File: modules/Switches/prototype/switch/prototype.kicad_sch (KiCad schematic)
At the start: 22 parts, among them J1 Conn_01x09, Q1 J109/J112, Q2 J109/J112, Q3 2N3906, SW2 SW_Push_LED, U1 TL072, U2 SN74HCS74

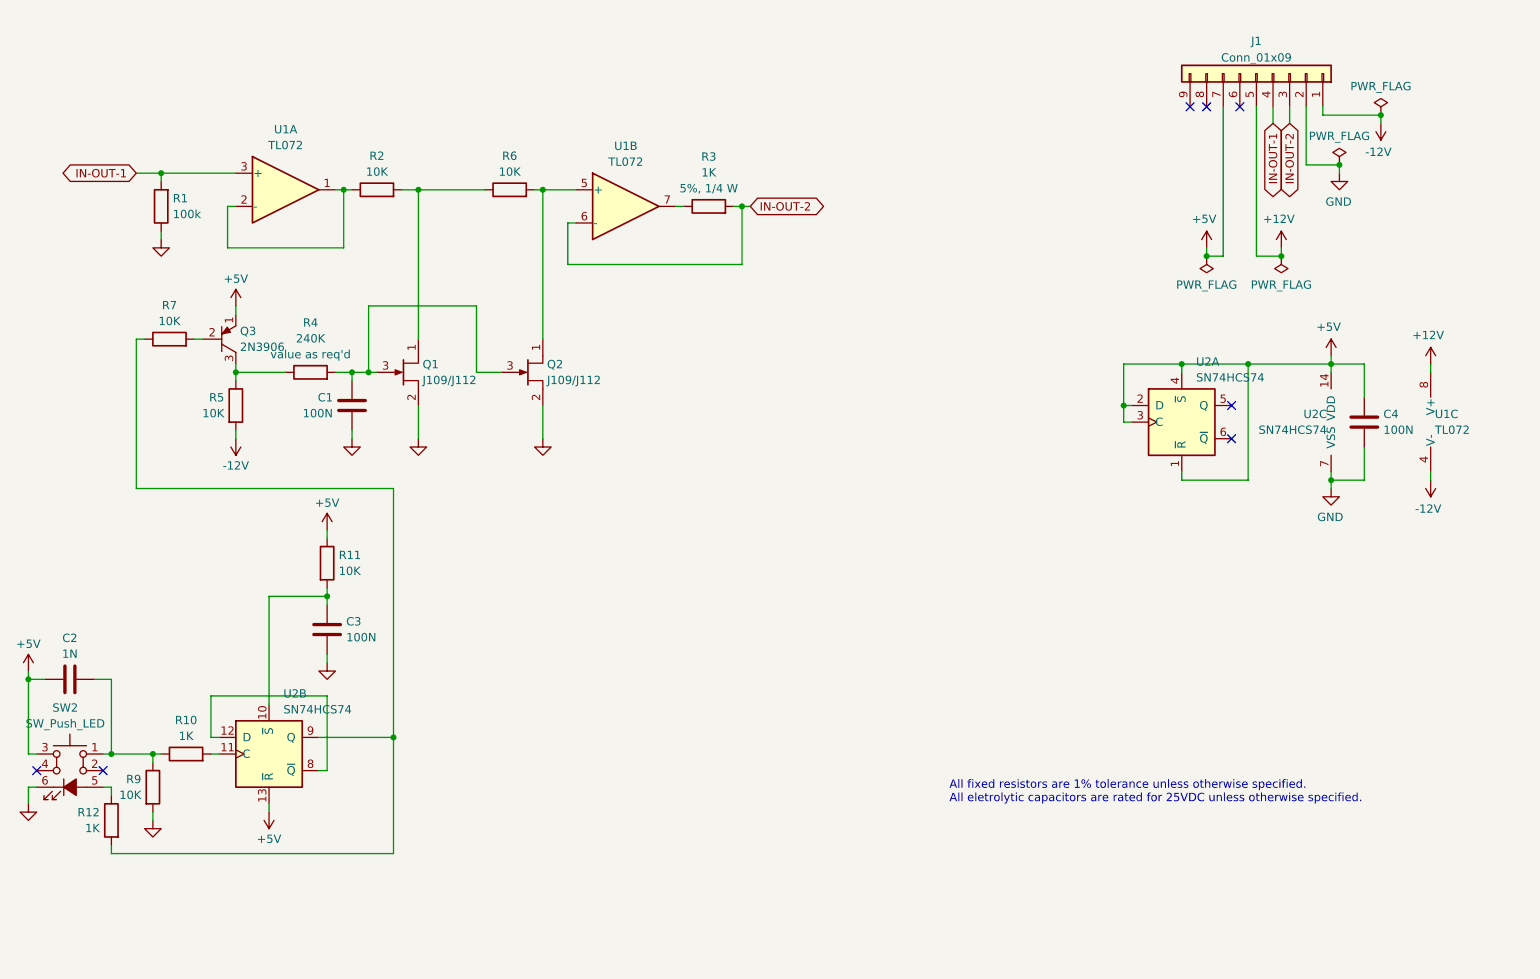
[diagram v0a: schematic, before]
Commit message: Switches - module design - wip
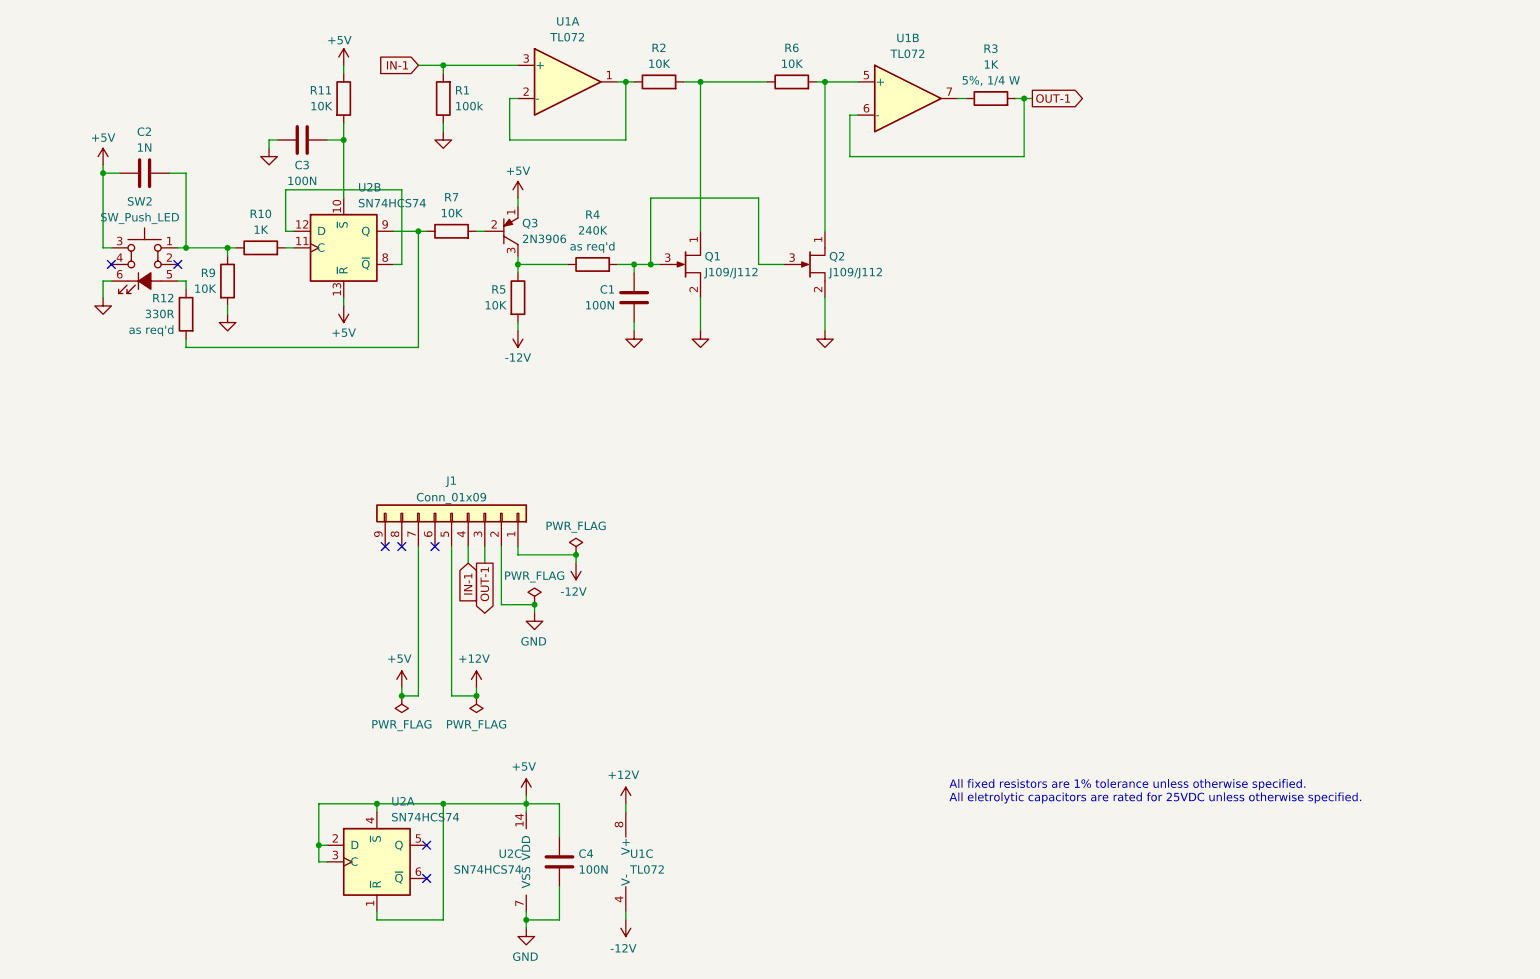
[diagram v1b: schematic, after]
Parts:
- R12: value 1K -> 330R; Note Output limiting -> as req'd
- R4: Note value as req'd -> as req'd
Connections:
- net IN-OUT-1 renamed IN-1
- net IN-OUT-2 renamed OUT-1
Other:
- moved on the sheet: C1, C2, C3, C4, J1, Q1, Q2, Q3, R1, R10, R11, R12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
